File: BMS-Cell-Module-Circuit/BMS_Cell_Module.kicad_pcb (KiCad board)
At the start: 2 copper layers, 64.1 x 62.7 mm, 38 parts, among them J1 Conn_01x02_Male, J2 Conn_01x04_Female, J3 Conn_01x04_Female, J4 Conn Female, J5 Conn Male, M1 SI2312BDS-T1-E3, U1 MCP1703A-3302_SOT223, U2 ADUM1250ARZ, U3 ATTINY85-20SU

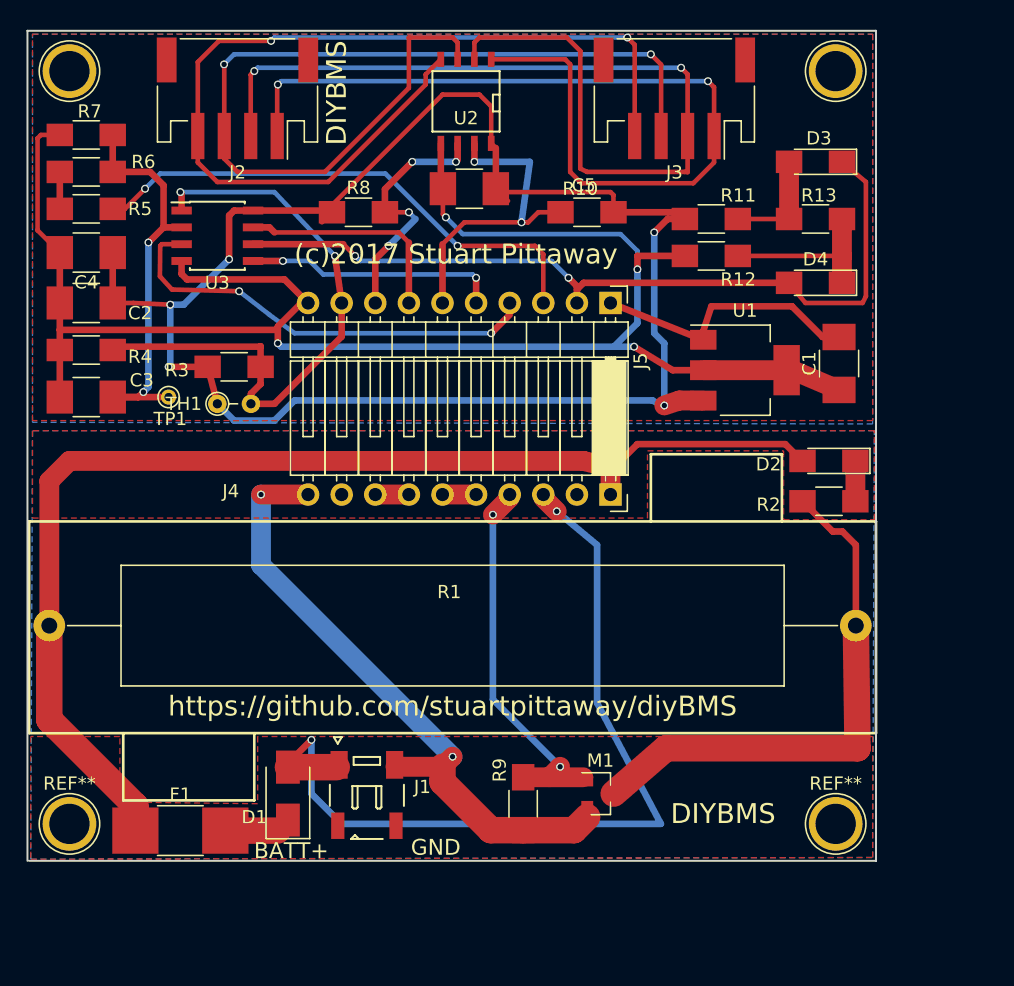
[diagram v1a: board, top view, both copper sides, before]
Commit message: Started redesign of PCB
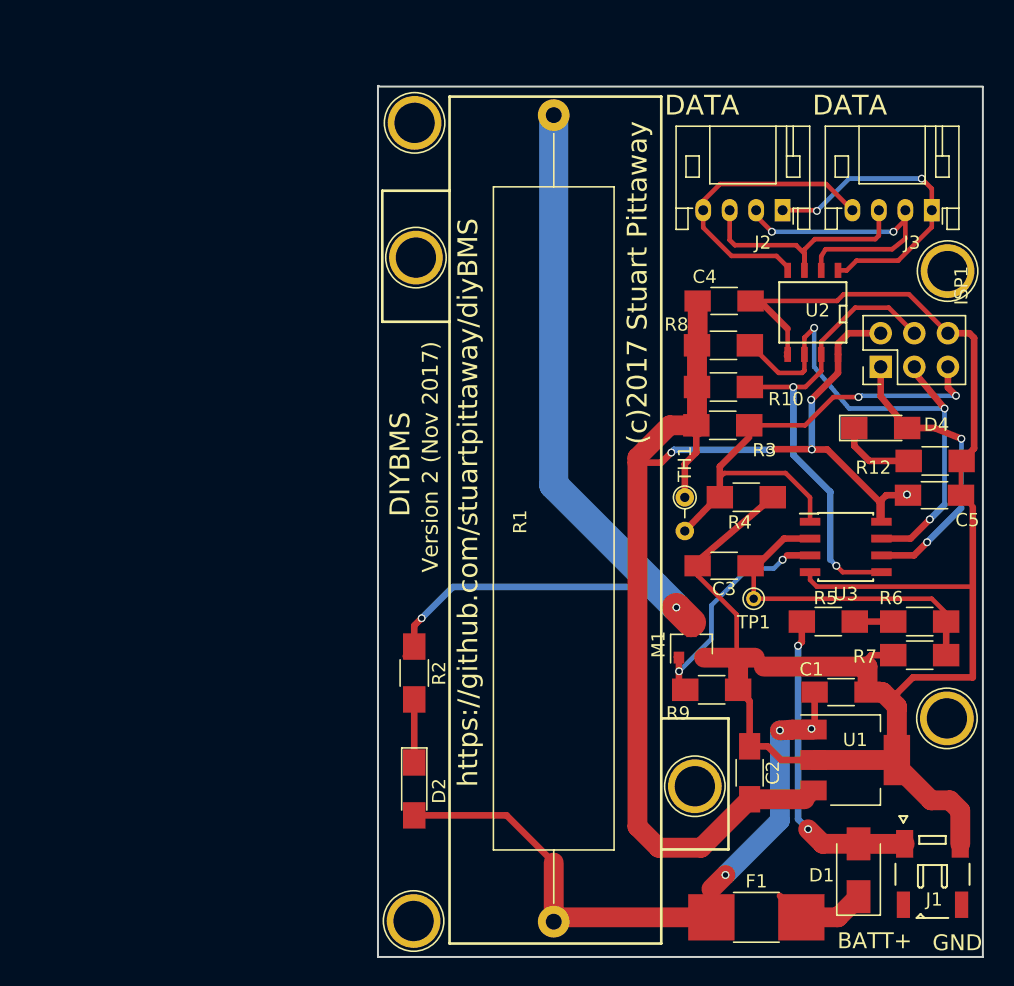
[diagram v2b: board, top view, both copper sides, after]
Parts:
- removed ? (x2): 1pin, Connectors:1pin
- removed D3: LED RED, LEDs:LED_1206_HandSoldering
- removed J4: Conn Female, Socket_Strips:Socket_Strip_Angled_1x10_Pitch2.54mm
- removed J5: Conn Male, Pin_Headers:Pin_Header_Angled_1x10_Pitch2.54mm
- removed R11: 510R, Resistors_SMD:R_1206_HandSoldering
- removed R13: 2K2, Resistors_SMD:R_1206_HandSoldering
- removed the REF** at (165.9, 116.1)
- removed the REF** at (108.0, 116.1)
- added ISP1: Conn_02x03_Odd_Even, Pin_Headers:Pin_Header_Straight_2x03_Pitch2.54mm, F.Cu at (169.3, 81.5)
- added REF**: 1pin, Connectors:1pin, F.Cu at (174.3, 74.3)
- added REF**: 1pin, Connectors:1pin, F.Cu at (174.3, 108.1)
- added REF**: 1pin, Connectors:1pin, F.Cu at (155.2, 113.2)
- added REF**: 1pin, Connectors:1pin, F.Cu at (134.1, 73.3)
- added REF**: 1pin, Connectors:1pin, F.Cu at (134.0, 63.1)
- added REF**: 1pin, Connectors:1pin, F.Cu at (134.0, 123.4)
- C1, C2: value 1uF -> 1uF Ceramic; footprint Capacitors_SMD:C_1210_HandSoldering -> Capacitors_SMD:C_1206_HandSoldering
- C3, C4, C5: footprint Capacitors_SMD:C_1210_HandSoldering -> Capacitors_SMD:C_1206_HandSoldering
- D2: value LED BLUE -> LED BLUE KPL-3015QBC-D
- J1: value Conn_01x02_Male -> Conn_01x02_Female
- J2, J3: footprint Connectors_JST:JST_PH_S4B-PH-SM4-TB_04x2.00mm_Angled -> Connectors_JST:JST_PH_S4B-PH-K_04x2.00mm_Angled
- R12: value 510R -> 2K2
- R2: value 47R 1/4W -> 47R
- moved R7 74.3 mm to (172.2, 103.3)
- moved R6 71.6 mm to (172.2, 100.8)
- moved R5 64.2 mm to (165.3, 100.8), turned to 0 degrees
- moved C2 61.4 mm to (159.4, 112.2), turned to 270 degrees
- moved U3 53.0 mm to (166.6, 95.1)
- moved R4 51.1 mm to (159.1, 91.4), turned to 0 degrees
- moved C3 49.9 mm to (157.4, 96.6)
- moved C4 48.3 mm to (157.4, 76.6), turned to 0 degrees
- moved TP1 46.8 mm to (159.7, 99.1)
- moved R1 44.8 mm to (144.6, 62.5), turned to 270 degrees
- moved F1 44.0 mm to (159.9, 123.1)
- moved D1 43.5 mm to (167.6, 119.6)
- moved J1 43.2 mm to (173.2, 119.9)
- moved C5 42.1 mm to (173.3, 91.2), turned to 0 degrees
- moved J2 42.1 mm to (161.8, 69.7)
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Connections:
- C1 pad 1: GND2 -> GND
- C2 pad 1: GND2 -> GND
- C3 pad 2: GND2 -> GND
- C4 pad 2: GND2 -> GND
- C5 pad 2: GND2 -> GND
- D2 pad 2: BATT+ -> Net-(C1-Pad2)
- F1 pad 1: BATT+ -> Net-(C1-Pad2)
- M1 pad 1: Net-(J4-Pad4) -> Net-(M1-Pad1)
- R1 pad 2: BATT+ -> Net-(C1-Pad2)
- R10 pad 1: Net-(J5-Pad6) -> Net-(ISP1-Pad4)
- R12 pad 2: GND2 -> GND
- R4 pad 2: GND2 -> GND
- R5 pad 1: Net-(J5-Pad3) -> BATT+RAW
- R7 pad 2: GND2 -> GND
- R8 pad 2: Net-(J5-Pad8) -> Net-(ISP1-Pad3)
- R9 pad 1: Net-(J4-Pad4) -> Net-(M1-Pad1)
- U1 pad 2: GND2 -> GND
- U2 pad 5: GND2 -> GND
- U2 pad 6: Net-(J5-Pad8) -> Net-(ISP1-Pad3)
- U2 pad 7: Net-(J5-Pad6) -> Net-(ISP1-Pad4)
- U3 pad 3: Net-(J5-Pad4) -> Net-(M1-Pad1)
- U3 pad 4: GND2 -> GND
- U3 pad 5: Net-(J5-Pad5) -> Net-(ISP1-Pad4)
- U3 pad 7: Net-(J5-Pad7) -> Net-(ISP1-Pad3)
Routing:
- net GND2: track 134.5 -> 0.00 mm, vias 4 -> 0
- net GND: track 49.0 -> 143.5 mm, vias 2 -> 0
- net BATT+: track 92.1 -> 0.00 mm
- net Net-(J2-Pad3): track 72.1 -> 19.2 mm, vias 2 -> 0
- net Net-(J2-Pad4): track 71.8 -> 22.5 mm, vias 2 -> 0
- net Net-(J2-Pad2): track 72.4 -> 23.5 mm
- net Net-(J2-Pad1): track 69.0 -> 24.0 mm
- net Net-(ISP1-Pad3): track 0.00 -> 41.2 mm, vias 0 -> 3
- net BATT+RAW: track 66.1 -> 25.5 mm
- net Net-(J5-Pad3): track 39.9 -> 0.00 mm, vias 2 -> 0
- net Net-(D4-Pad2): track 62.2 -> 22.7 mm
- net Net-(ISP1-Pad4): track 0.00 -> 36.7 mm, vias 0 -> 2
- net Net-(J5-Pad4): track 33.4 -> 0.00 mm, vias 2 -> 0
- net Net-(C1-Pad2): track 20.8 -> 53.8 mm, vias 0 -> 3
- net Net-(J4-Pad4): track 31.3 -> 0.00 mm, vias 2 -> 0
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- removed copper zone on B.Cu, net GND
- removed copper zone on F.Cu, net GND
- removed copper zone on B.Cu, net GND2
- removed copper zone on F.Cu, net GND2
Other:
- board size 64.1 x 62.7 mm -> 45.7 x 65.8 mm
- board text added: "DATA"
- board text added: "Version 2 (Nov 2017)"
